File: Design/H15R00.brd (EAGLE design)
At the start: 34.6 x 30 mm, 36 parts, among them P1 HEXABIT_17.32_NO_P3_P6, U1 STM32F091CBU6, U2 OPA188, X1 XTALL_CSTCE8M00G52

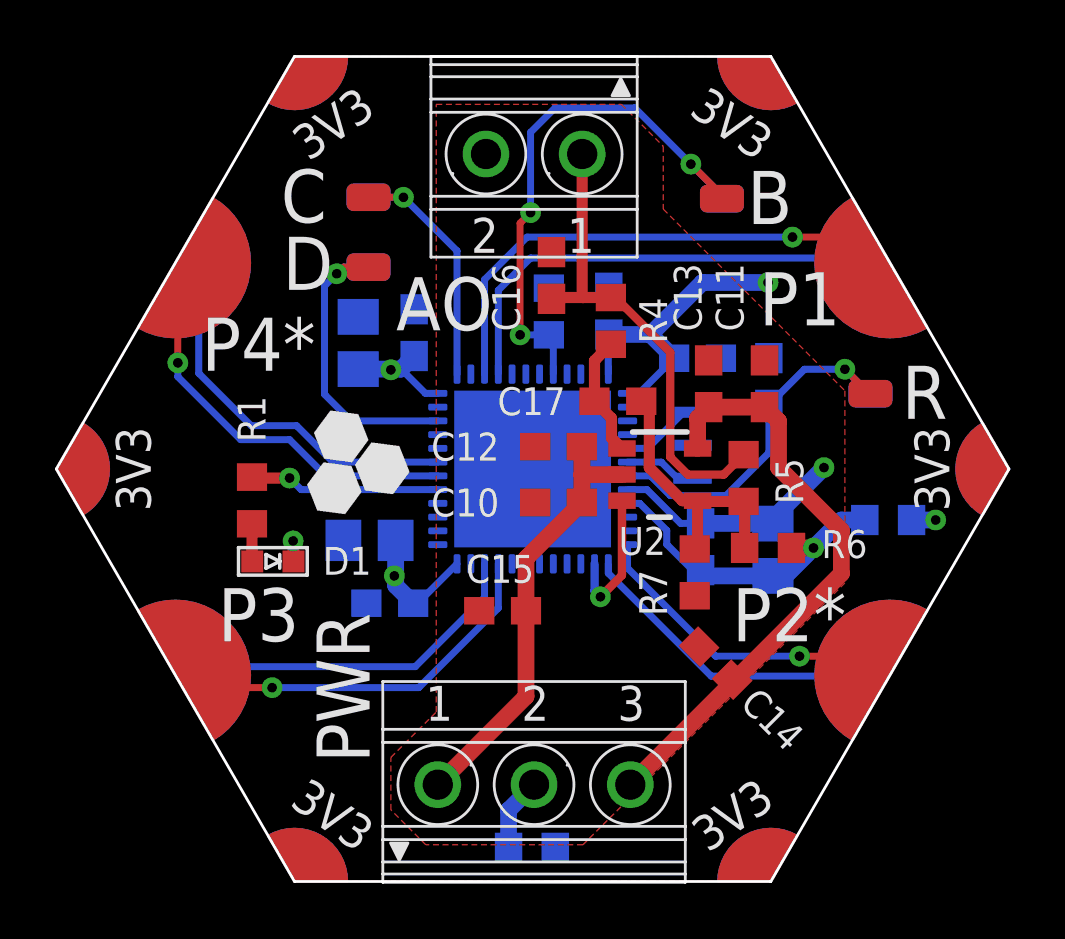
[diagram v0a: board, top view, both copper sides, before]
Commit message: Solved DRC Generated gerber, drill, pick n place and schematics Generated BOM First release Ver 0
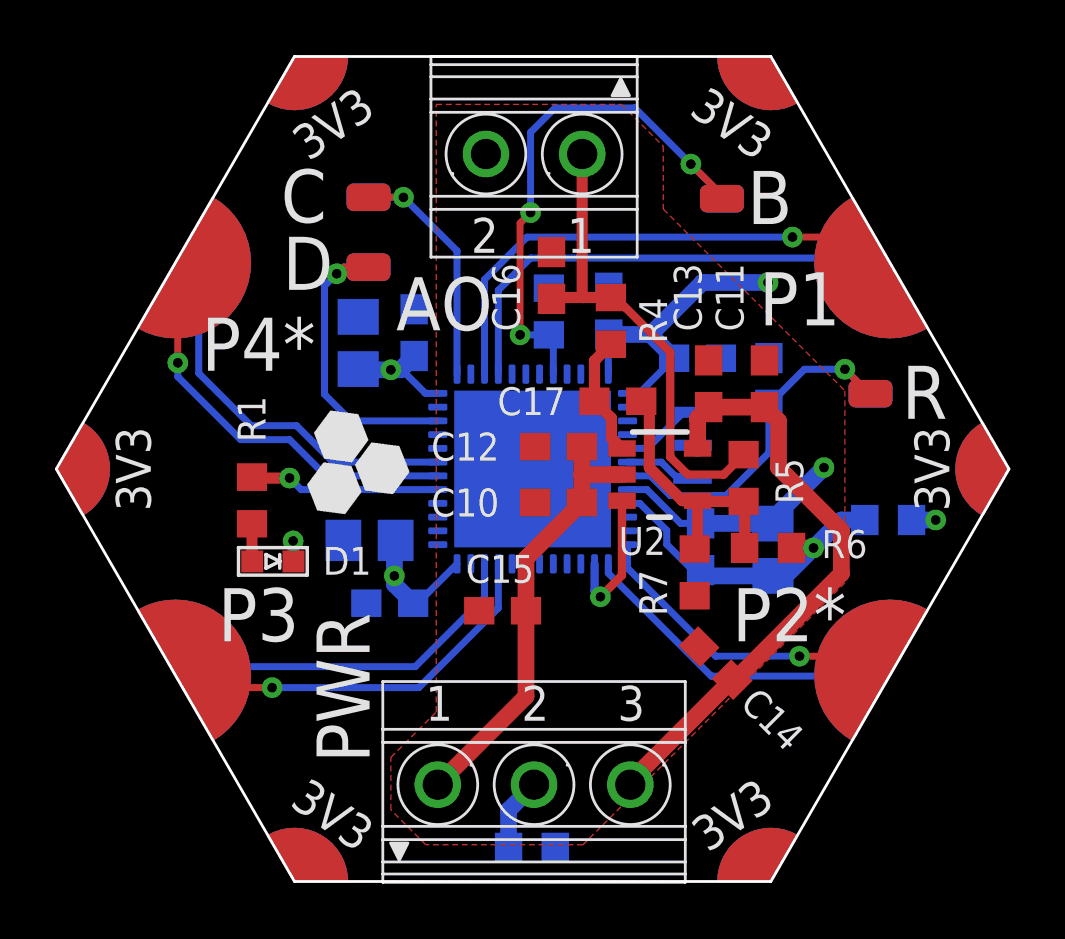
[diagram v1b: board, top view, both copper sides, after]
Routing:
- net VDD: track 21.0 -> 21.7 mm
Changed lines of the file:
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@@
 <attribute name="COMPTYPE" value="IC" x="39.243" y="34.417" size="1.778" layer="27" display="off"/>
 <attribute name="MANUFACTURER" value="Texas Instruments" x="39.243" y="34.417" size="1.778" layer="27" display="off"/>
+<attribute name="MFN" value="Texas Instruments" x="39.243" y="34.417" size="1.778" layer="27" display="off"/>
 <attribute name="MOUNTTYPE" value="SMT" x="39.243" y="34.417" size="1.778" layer="27" display="off"/>
+<attribute name="MPN" value="OPA188AIDBVR" x="39.243" y="34.417" size="1.778" layer="27" display="off"/>
 <attribute name="NAME" x="37.7444" y="31.496" size="1.016" layer="25" rot="SR0"/>
+<attribute name="OCTOPART_URL" value="https://octopart.com/opa188aidbvr-texas+instruments-27810397?r=sp&amp;s=zwpAzK6tSwu39ID1-8lLKg" x="39.243" y="34.417" size="1.778" layer="27" display="off"/>
 <attribute name="PACKAGEREFERENCE" value="DBV0005A" x="39.243" y="34.417" size="1.778" layer="27" display="off"/>
 <attribute name="PARTNUMBER" value="OPA188AIDBVR" x="39.243" y="34.417" size="1.778" layer="27" display="off"/>
@@
 <attribute name="NAME" x="38.493190625" y="30.94939375" size="1.016" layer="25" rot="R270"/>
 <attribute name="OCTOPART_URL" value="https://octopart.com/era-3aeb1242v-panasonic-55639351?r=sp&amp;s=K0xQjqOwSGaT1tqbXnh0hg" x="40.513" y="30.861" size="1.778" layer="27" rot="R270" display="off"/>
-<attribute name="RESISTANCE" value="12.4 Ohm" x="40.513" y="30.861" size="1.778" layer="27" rot="R270" display="off"/>
+<attribute name="RESISTANCE" value="12.4 kOhm" x="40.513" y="30.861" size="1.778" layer="27" rot="R270" display="off"/>
 <attribute name="TOLERANCE" value="0.1%" x="40.513" y="30.861" size="1.778" layer="27" rot="R270" display="off"/>
 <attribute name="VALUE" x="38.622984375" y="32.398971875" size="1.016" layer="27" rot="R270"/>
@@
 <wire x1="31.8702" y1="31.17019375" x2="30.44035625" y2="29.74035" width="0.254" layer="16"/>
 <wire x1="30.44035625" y1="29.74035" x2="30.274375" y2="29.74035" width="0.254" layer="16"/>
-<wire x1="30.274375" y1="29.74035" x2="29.638284375" y2="30.376440625" width="0.6096" layer="16"/>
-<wire x1="29.638284375" y1="30.376440625" x2="29.638284375" y2="32.022790625" width="0.6096" layer="16"/>
-<wire x1="28.276303125" y1="38.253853125" x2="29.8359" y2="38.253853125" width="0.6096" layer="16"/>
 <wire x1="29.8359" y1="38.253853125" x2="30.3095625" y2="38.727515625" width="0.6096" layer="16"/>
 <wire x1="31.17019375" y1="37.3702" x2="30.719553125" y2="37.3702" width="0.254" layer="16"/>
@@
 <wire x1="40.7904875" y1="41.402" x2="43.18" y2="41.402" width="0.6096" layer="16"/>
 <via x="43.18" y="41.402" extent="1-16" drill="0.35"/>
-<wire x1="29.464" y1="38.227" x2="29.8359" y2="38.253853125" width="0" layer="19" extent="16-16"/>
-<wire x1="29.638284375" y1="30.376440625" x2="29.591" y2="30.734" width="0" layer="19" extent="16-16"/>
+<wire x1="30.3095625" y1="38.727515625" x2="29.809046875" y2="38.227" width="0.6096" layer="16"/>
+<wire x1="29.809046875" y1="38.227" x2="29.464" y2="38.227" width="0.6096" layer="16"/>
+<wire x1="29.464" y1="38.227" x2="28.30315625" y2="38.227" width="0.6096" layer="16"/>
+<wire x1="28.30315625" y1="38.227" x2="28.276303125" y2="38.253853125" width="0.6096" layer="16"/>
+<wire x1="29.591" y1="30.734" x2="29.591" y2="30.423725" width="0.6096" layer="16"/>
+<wire x1="29.591" y1="30.423725" x2="30.274375" y2="29.74035" width="0.6096" layer="16"/>
+<wire x1="29.591" y1="30.734" x2="29.591" y2="31.97550625" width="0.6096" layer="16"/>
+<wire x1="29.591" y1="31.97550625" x2="29.638284375" y2="32.022790625" width="0.6096" layer="16"/>
 </signal>
 <signal name="UART3_TX">
@@
 <wire x1="40.618" y1="36.466" x2="41.021" y2="36.869" width="0.6096" layer="1"/>
 <wire x1="41.021" y1="36.869" x2="43.053" y2="36.869" width="0.6096" layer="1"/>
-<wire x1="38.171" y1="23.141" x2="45.847" y2="30.817" width="0.6096" layer="1"/>
-<wire x1="45.847" y1="30.817" x2="45.847" y2="32.385" width="0.6096" layer="1"/>
+<wire x1="45.847" y1="32.385" x2="45.847" y2="30.817" width="0.6096" layer="1"/>
 <wire x1="45.847" y1="32.385" x2="43.561" y2="34.671" width="0.6096" layer="1"/>
 <wire x1="43.053" y1="36.869" x2="43.561" y2="36.361" width="0.6096" layer="1"/>
 <wire x1="43.561" y1="36.361" x2="43.561" y2="34.671" width="0.6096" layer="1"/>
-<wire x1="38.171" y1="23.141" x2="41.876040625" y2="26.95795625" width="0" layer="19" extent="1-1"/>
+<wire x1="45.847" y1="30.817" x2="41.98795625" y2="26.95795625" width="0.6096" layer="1"/>
+<wire x1="41.98795625" y1="26.95795625" x2="41.876040625" y2="26.95795625" width="0.6096" layer="1"/>
+<wire x1="41.876040625" y1="26.95795625" x2="38.171" y2="23.252915625" width="0.6096" layer="1"/>
+<wire x1="38.171" y1="23.252915625" x2="38.171" y2="23.141" width="0.6096" layer="1"/>
 </signal>
 <signal name="-15V">
@@
 <mfgpreviewcolor name="substratecolor" color="0xFF786E46"/>
 </mfgpreviewcolors>
+<errors>
+</errors>
 </board>
 </drawing>
